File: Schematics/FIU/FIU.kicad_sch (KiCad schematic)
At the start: 2 parts

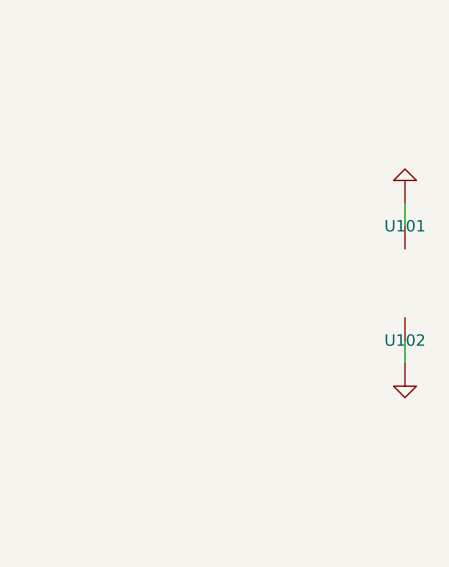
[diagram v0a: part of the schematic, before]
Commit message: Snapshot.
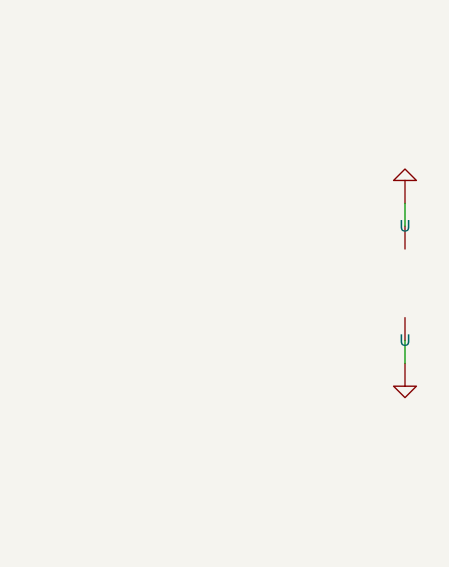
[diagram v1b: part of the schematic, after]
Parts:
- renumbered U102 to U, U101 to U
